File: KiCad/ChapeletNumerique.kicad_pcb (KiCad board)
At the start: 2 copper layers, 26 parts

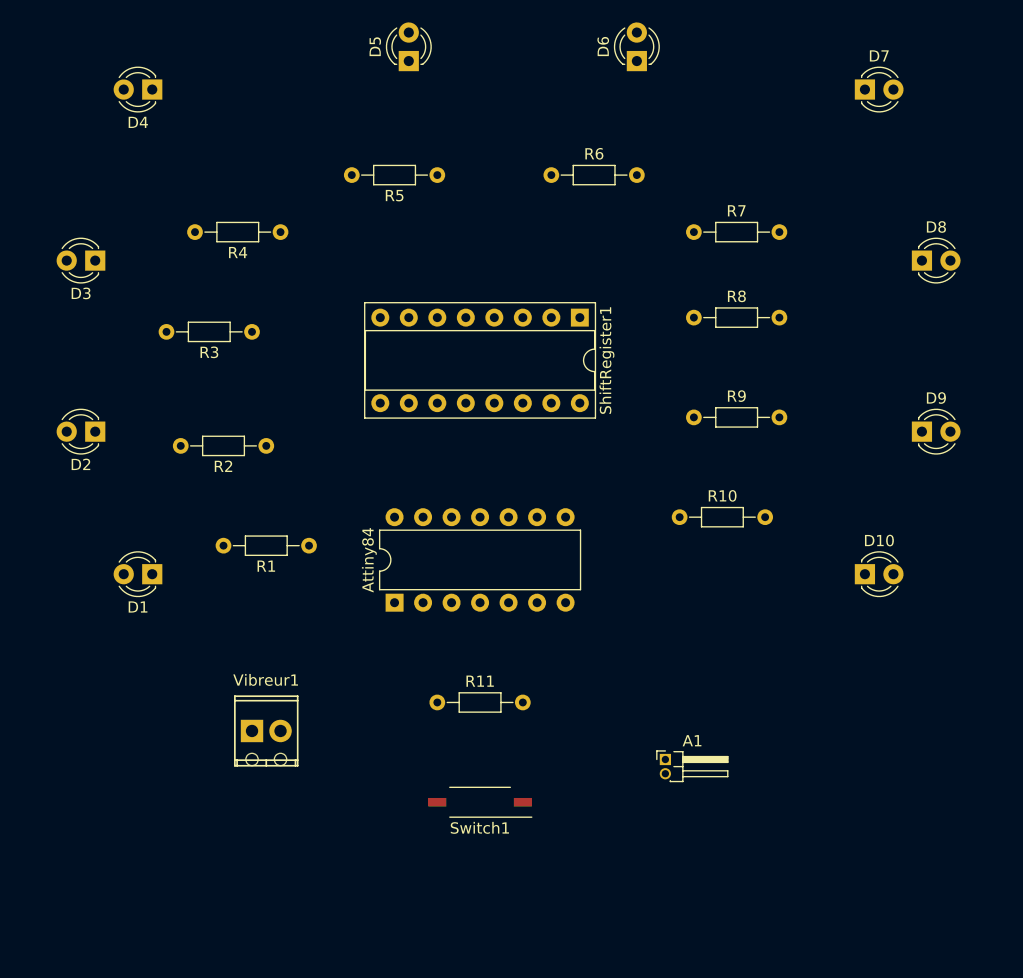
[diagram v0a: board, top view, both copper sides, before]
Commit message: fear(kicad) PCB finished
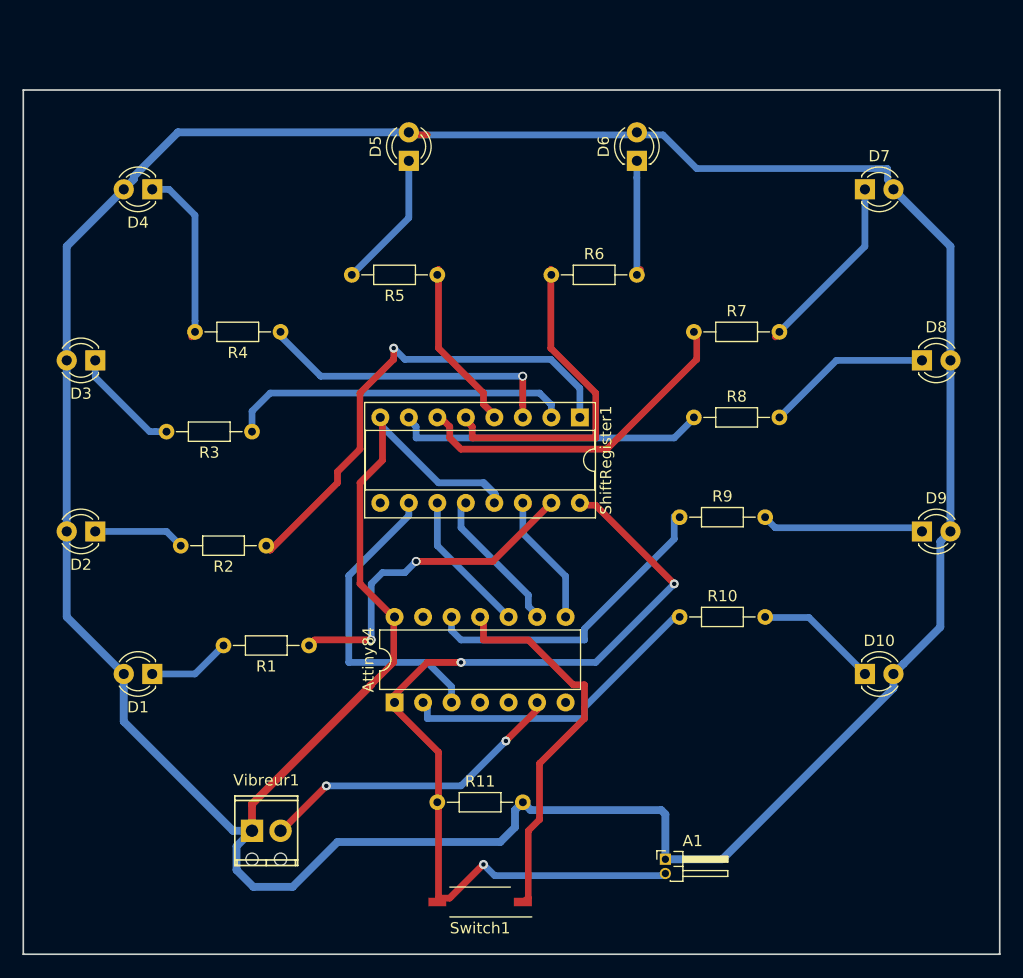
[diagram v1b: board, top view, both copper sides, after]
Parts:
- moved R9 8.98 mm to (157.5, 99.1)
- moved D1 8.89 mm to (110.5, 113.0)
- moved D10 8.89 mm to (174.0, 113.0)
- moved D2 8.89 mm to (105.4, 100.3)
- moved D3 8.89 mm to (105.4, 85.1)
- moved D5 8.89 mm to (133.3, 67.3)
- moved D6 8.89 mm to (153.7, 67.3)
- moved D8 8.89 mm to (179.1, 85.1)
- moved D9 8.89 mm to (179.1, 100.3)
- moved R1 8.89 mm to (124.5, 110.5)
- moved R10 8.89 mm to (157.5, 108.0)
- moved R11 8.89 mm to (135.9, 124.5)
- moved R2 8.89 mm to (120.7, 101.6)
- moved R3 8.89 mm to (119.4, 91.4)
- moved R4 8.89 mm to (121.9, 82.5)
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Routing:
- net GND: track 0.00 -> 336.8 mm
- net VCC: track 0.00 -> 84.7 mm, vias 0 -> 3
- net Net-(R2-Pad1): track 0.00 -> 43.7 mm, vias 0 -> 1
- net /switch: track 0.00 -> 34.6 mm
- net Net-(R6-Pad1): track 0.00 -> 31.0 mm
- net Net-(R3-Pad1): track 0.00 -> 30.9 mm
- net Net-(R7-Pad1): track 0.00 -> 30.9 mm
- net Net-(R1-Pad1): track 0.00 -> 30.0 mm, vias 0 -> 2
- net Net-(Attiny84-Pad3): track 0.00 -> 29.8 mm
- net Net-(R8-Pad1): track 0.00 -> 28.9 mm
- net Net-(Attiny84-Pad2): track 0.00 -> 28.4 mm
- net Net-(Attiny84-Pad12): track 0.00 -> 28.2 mm
- net Net-(Attiny84-Pad6): track 0.00 -> 28.1 mm, vias 0 -> 2
- net Net-(R4-Pad1): track 0.00 -> 27.1 mm, vias 0 -> 1
- net Net-(D7-Pad1): track 0.00 -> 16.6 mm
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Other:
- board outline added: 87 x 77 mm
- net class Alimentation added: clearance 0.2, trace_width 0.7, via_dia 1, via_drill 0.5
- net class Default: trace_width 0.25 -> 0.6; via_dia 0.6 -> 0.8; via_drill 0.4 -> 0.5
